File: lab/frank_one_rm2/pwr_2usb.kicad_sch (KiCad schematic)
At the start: 39 parts, among them J13 USB4215-03-A, J14 USB4215-03-A, U10 ME6211C33M5, U11 ME6211C18M5, U6 USBLC6-2SC6, U7 USBLC6-2SC6, U8 ME6211C33M5, U9 ME6211C33M5

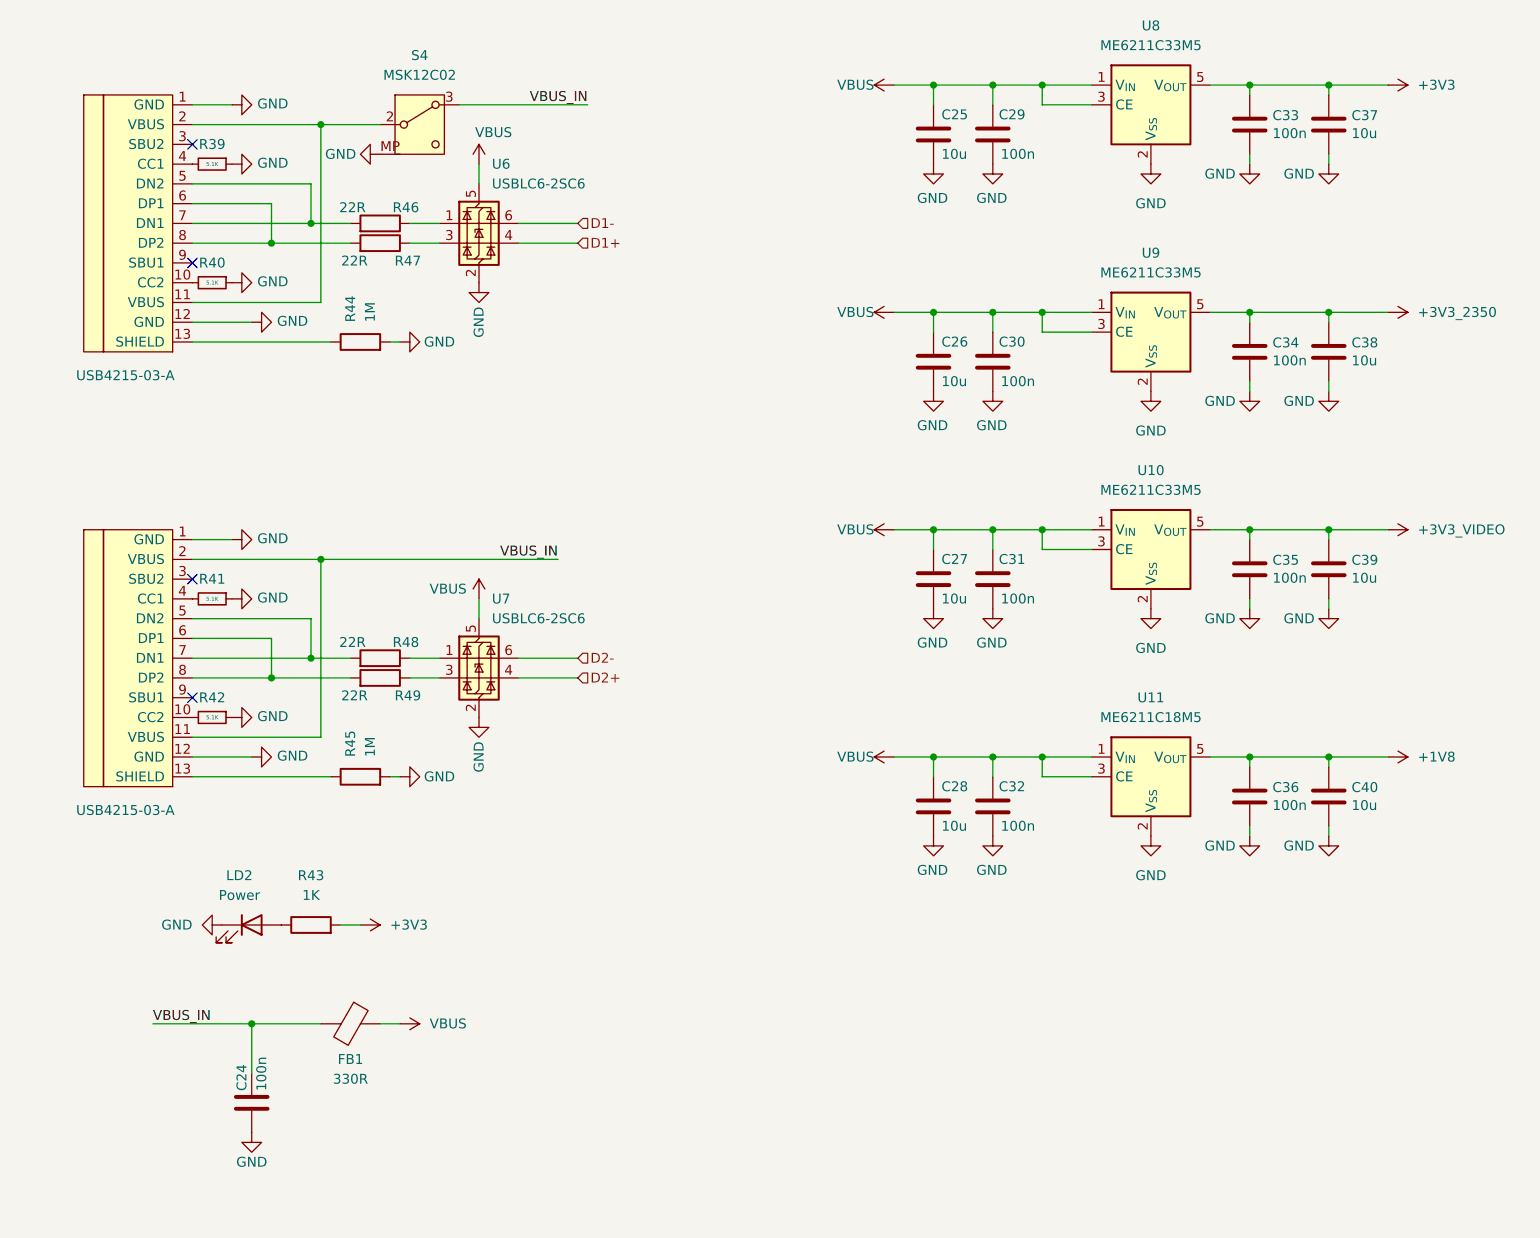
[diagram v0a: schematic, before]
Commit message: FRANK One RM2 HW 1.03
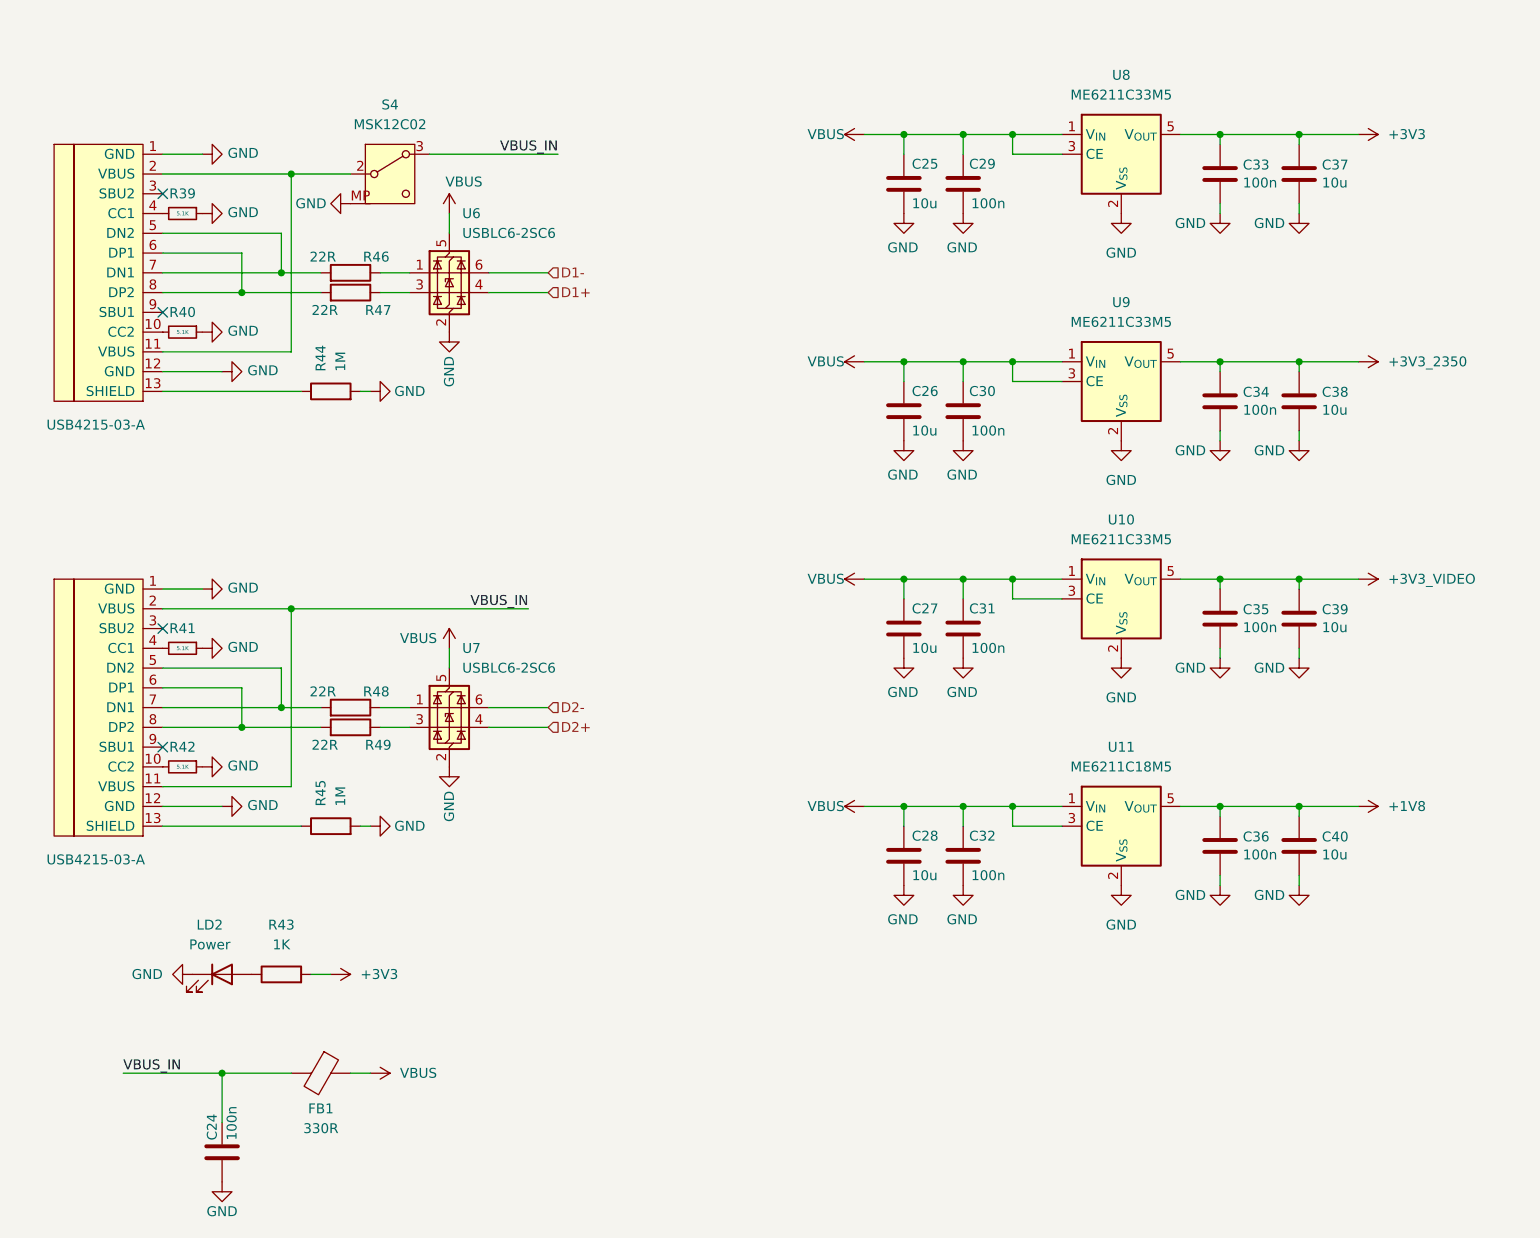
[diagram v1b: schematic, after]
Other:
- moved on the sheet: C24, C25, C26, C27, C28, C29, C30, C31, C32, C33, C34, C35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
